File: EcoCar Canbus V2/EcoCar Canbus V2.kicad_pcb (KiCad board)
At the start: 2 copper layers, 112.5 x 50 mm, 11 parts

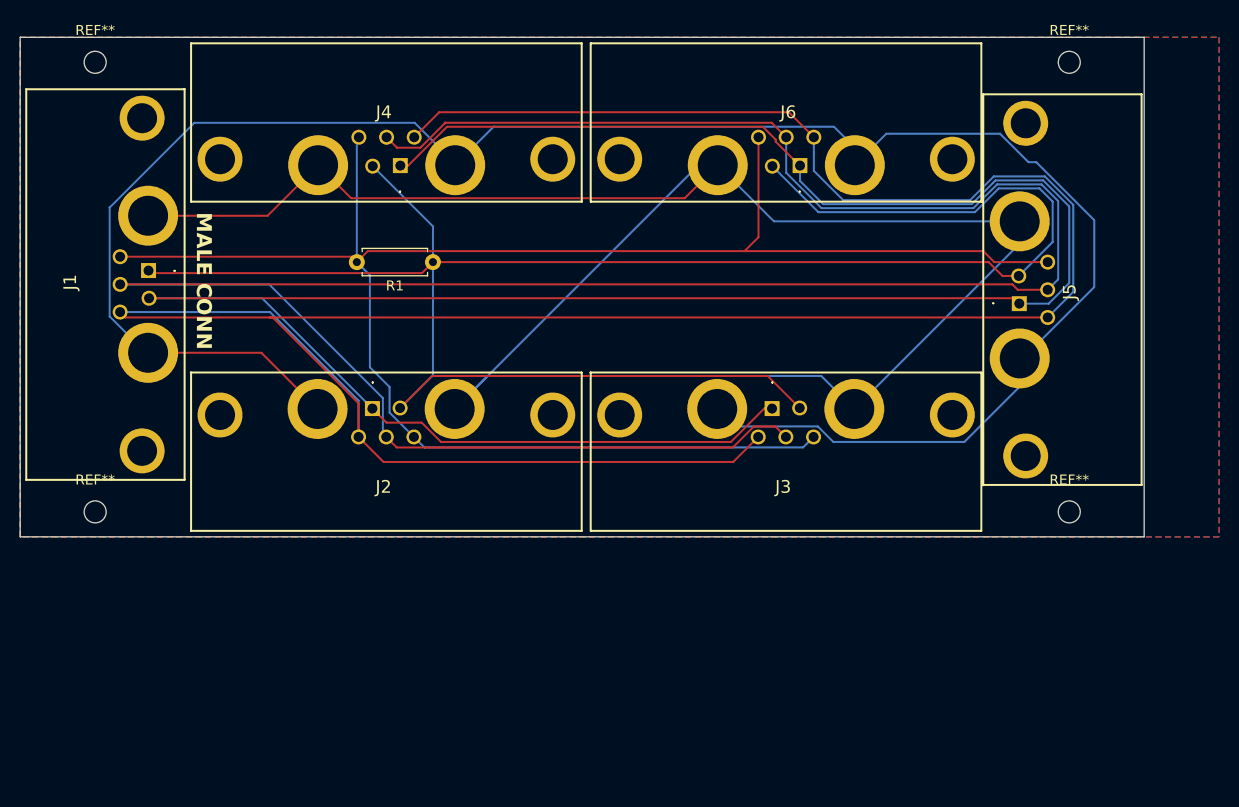
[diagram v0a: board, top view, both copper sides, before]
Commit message: Changed connectors,footprints,pinouts. Almost ready :)
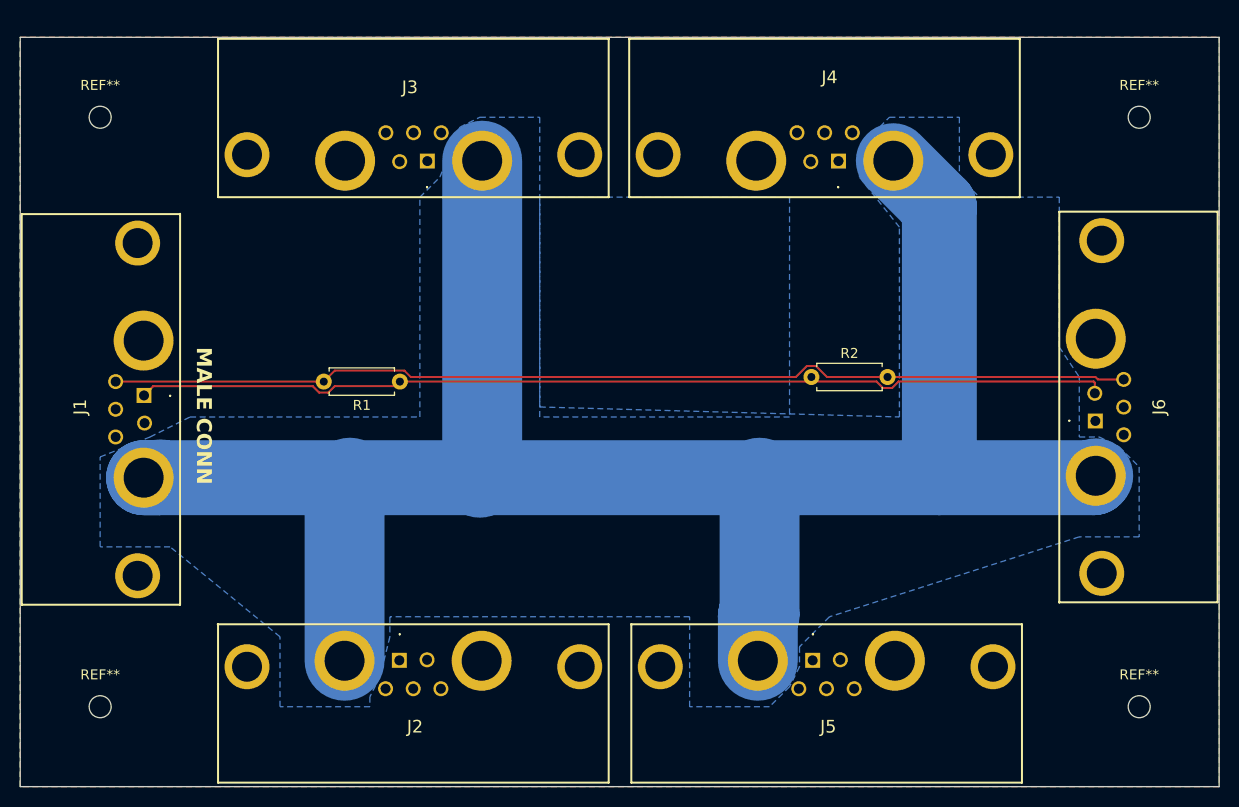
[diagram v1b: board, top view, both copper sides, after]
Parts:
- added R2: 120, Resistor_THT:R_Axial_DIN0207_L6.3mm_D2.5mm_P7.62mm_Horizontal, F.Cu at (154.2, 84.0)
- moved J3 46.6 mm to (114.4, 60.8), turned to 180 degrees
- moved J5 44.0 mm to (155.7, 114.0), turned to 0 degrees
- moved J4 43.9 mm to (155.5, 60.8)
- moved J6 41.5 mm to (184.2, 87.0), turned to 90 degrees
- moved J2 25.3 mm to (114.3, 114.0)
- moved REF** 20.7 mm to (187.0, 117.0)
- moved REF** 19.5 mm to (83.0, 117.0)
- moved J1 12.5 mm to (85.8, 87.2)
- moved R1 12.4 mm to (113.0, 84.5)
- moved REF** 8.90 mm to (187.0, 58.0)
- moved REF** 5.52 mm to (83.0, 58.0)
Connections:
- net Net-(J1-Pad2) renamed 7V
- net Net-(J1-Pad3) renamed CAN-
- net Net-(J1-Pad6) renamed CAN+
- J1 pad 4: Net-(J1-Pad4) -> 12V
- J1 pad 5: Net-(J1-Pad5) -> 12V
- J1 pad 7: Net-(J1-Pad7) -> 12V
- J2 pad 3: Net-(J1-Pad5) -> 12V
- J2 pad 4: Net-(J1-Pad4) -> 12V
- J2 pad 6: Net-(J1-Pad7) -> 12V
- J3 pad 3: Net-(J1-Pad5) -> 12V
- J3 pad 4: Net-(J1-Pad4) -> 12V
- J3 pad 6: Net-(J1-Pad7) -> 12V
- J4 pad 3: Net-(J1-Pad5) -> 12V
- J4 pad 4: Net-(J1-Pad4) -> 12V
- J4 pad 6: Net-(J1-Pad7) -> 12V
- J5 pad 3: Net-(J1-Pad5) -> 12V
- J5 pad 4: Net-(J1-Pad4) -> 12V
- J5 pad 6: Net-(J1-Pad7) -> 12V
- J6 pad 3: Net-(J1-Pad5) -> 12V
- J6 pad 4: Net-(J1-Pad4) -> 12V
- J6 pad 6: Net-(J1-Pad7) -> 12V
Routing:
- net 12V: track 0.00 -> 414.2 mm
- net Net-(J1-Pad5): track 269.2 -> 0.00 mm
- net Net-(J1-Pad4): track 255.2 -> 0.00 mm
- net Net-(J1-Pad7): track 245.4 -> 0.00 mm
- net GND: track 199.2 -> 0.00 mm
- net CAN-: track 180.0 -> 227.4 mm
- net CAN+: track 199.3 -> 216.0 mm
- net 7V: track 202.5 -> 199.5 mm
- added copper zone on B.Cu, net 7V
- added copper zone on B.Cu, net GND
- added copper zone on F.Cu, net GND
- added copper zone on In1.Cu, net GND
- added copper zone on In2.Cu, net GND
- removed copper zone on B.Cu, net (none)
- removed copper zone on F.Cu, net (none)
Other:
- board size 112.5 x 50 mm -> 120 x 75 mm
- copper layers 2 -> 4
